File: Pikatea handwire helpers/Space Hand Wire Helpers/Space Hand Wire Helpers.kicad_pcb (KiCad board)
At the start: 2 copper layers, 104.9 x 20 mm, 3 parts

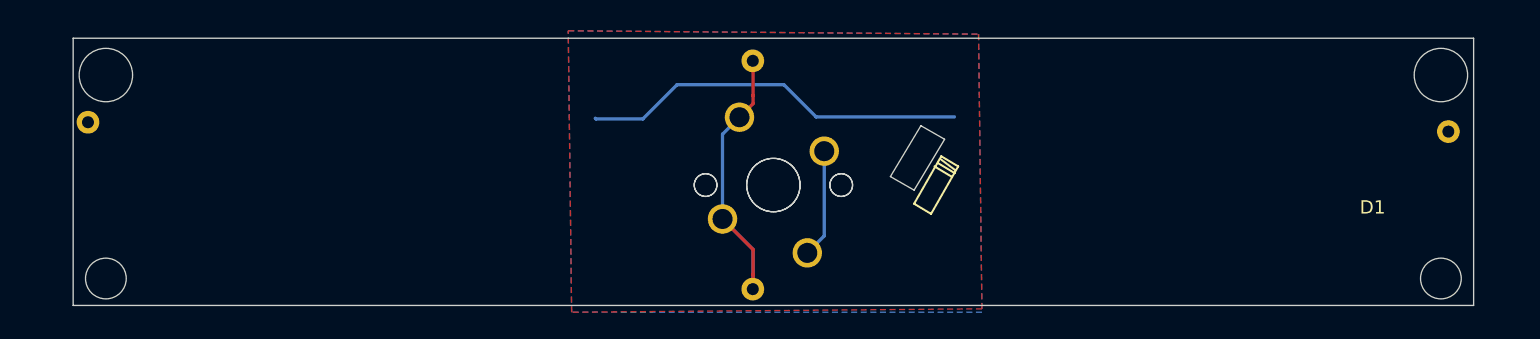
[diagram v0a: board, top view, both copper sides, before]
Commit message: update andwire gerbers
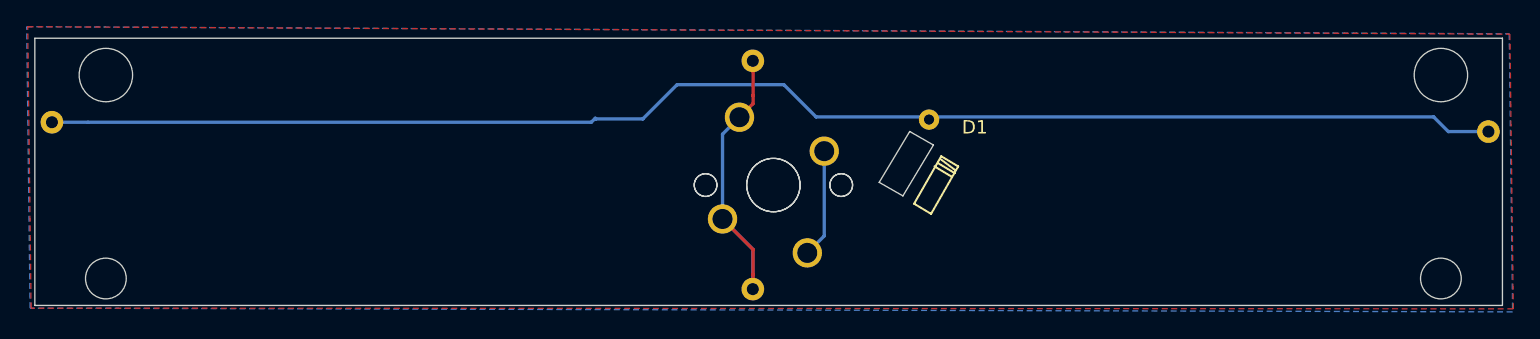
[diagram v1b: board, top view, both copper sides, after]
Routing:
- net Net-(D1-Pad1): track 29.0 -> 110.3 mm
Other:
- board size 104.9 x 20 mm -> 109.9 x 20 mm
